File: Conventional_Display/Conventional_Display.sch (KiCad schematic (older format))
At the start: 93 parts, among them J1 Conn_01x05_Female, U1 7-Segment_Display_CA, U10 7-Segment_Display_CA, U11 7-Segment_Display_CA, U12 7-Segment_Display_CA, U13 7-Segment_Display_CA, U14 7-Segment_Display_CA, U15 7-Segment_Display_CA, U16 MAX_7219, U17 MAX_7219, U18 MAX_7219, U19 MAX_7219, U2 7-Segment_Display_CA, U20 1088A5_8x8_LED_Matrix, U21 1088A5_8x8_LED_Matrix, U22 1088A5_8x8_LED_Matrix, U23 1088A5_8x8_LED_Matrix, U3 7-Segment_Display_CA, U4 7-Segment_Display_CA, U5 7-Segment_Display_CA, U6 7-Segment_Display_CA, U7 7-Segment_Display_CA, U8 7-Segment_Display_CA, U9 7-Segment_Display_CA

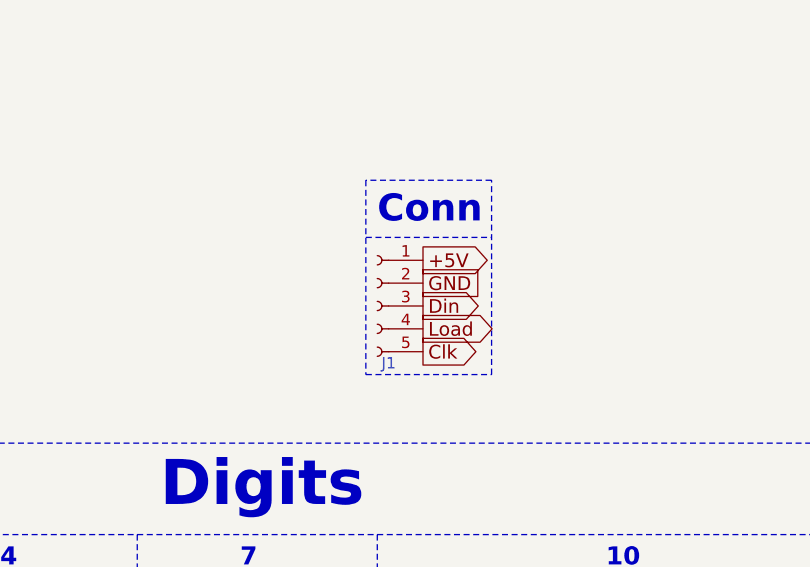
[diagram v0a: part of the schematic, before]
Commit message: Changes
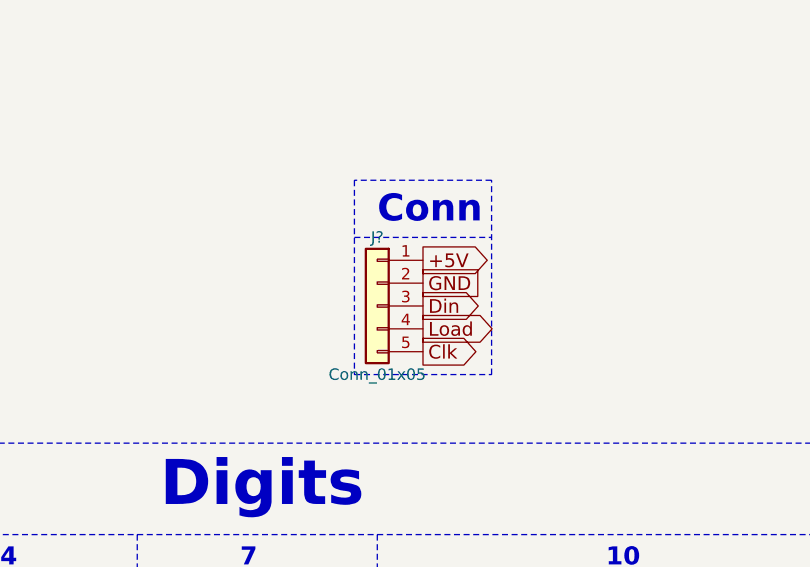
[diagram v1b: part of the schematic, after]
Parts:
- removed J1: Conn_01x05_Female, MRDT_Connectors:MOLEX_SL_5_Horizontal, symbol Conn_01x05_Female
- added J?: Conn_01x05, symbol Conn_01x05
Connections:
- net +5V: now also J?.1 (Pin_1)
- net Clk: now also J?.5 (Pin_5)
- net Din: now also J?.3 (Pin_3)
- net GND: now also J?.2 (Pin_2)
- net Load: now also J?.4 (Pin_4)
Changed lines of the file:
@@
 $EndDescr
-$Comp
-L Conn_01x05_Female J1
-U 1 1 5B441E73
-P 4300 3750
-F 0 "J1" H 4250 3500 50  0000 C CNN
-F 1 "Conn_01x05_Female" H 4300 3450 50  0001 C CNN
-F 2 "MRDT_Connectors:MOLEX_SL_5_Horizontal" H 4300 3750 50  0001 C CNN
-F 3 "" H 4300 3750 50  0001 C CNN
-	1    4300 3750
-	-1   0    0    -1
-$EndComp
 $Comp
 L 1088A5_8x8_LED_Matrix U20
@@
 Conn
 Wire Notes Line
-	4250 4050 4800 4050
+	4200 4050 4800 4050
 Wire Notes Line
 	4800 4050 4800 3200
 Wire Notes Line
-	4800 3200 4250 3200
-Wire Notes Line
-	4250 3200 4250 4050
-Wire Notes Line
-	4250 3450 4800 3450
+	4800 3200 4200 3200
+Wire Notes Line
+	4200 3450 4800 3450
 Wire Wire Line
 	1700 5050 1700 5100
@@
 Wire Wire Line
 	5950 7650 5950 7700
+Wire Notes Line
+	4200 3200 4200 4050
+$Comp
+L Conn_01x05 J?
+U 1 1 5B6CA188
+P 4300 3750
+F 0 "J?" H 4300 4050 50  0000 C CNN
+F 1 "Conn_01x05" H 4300 3450 50  0000 C CNN
+F 2 "" H 4300 3750 50  0001 C CNN
+F 3 "" H 4300 3750 50  0001 C CNN
+	1    4300 3750
+	-1   0    0    -1
+$EndComp
 $EndSCHEMATC
